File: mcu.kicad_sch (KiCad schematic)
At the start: 22 parts, among them J2 DM3CS-SF, J4 SCREEN, U4 ESP32-S3-WROOM-1U-N16R8, U8 SiP32431DR3

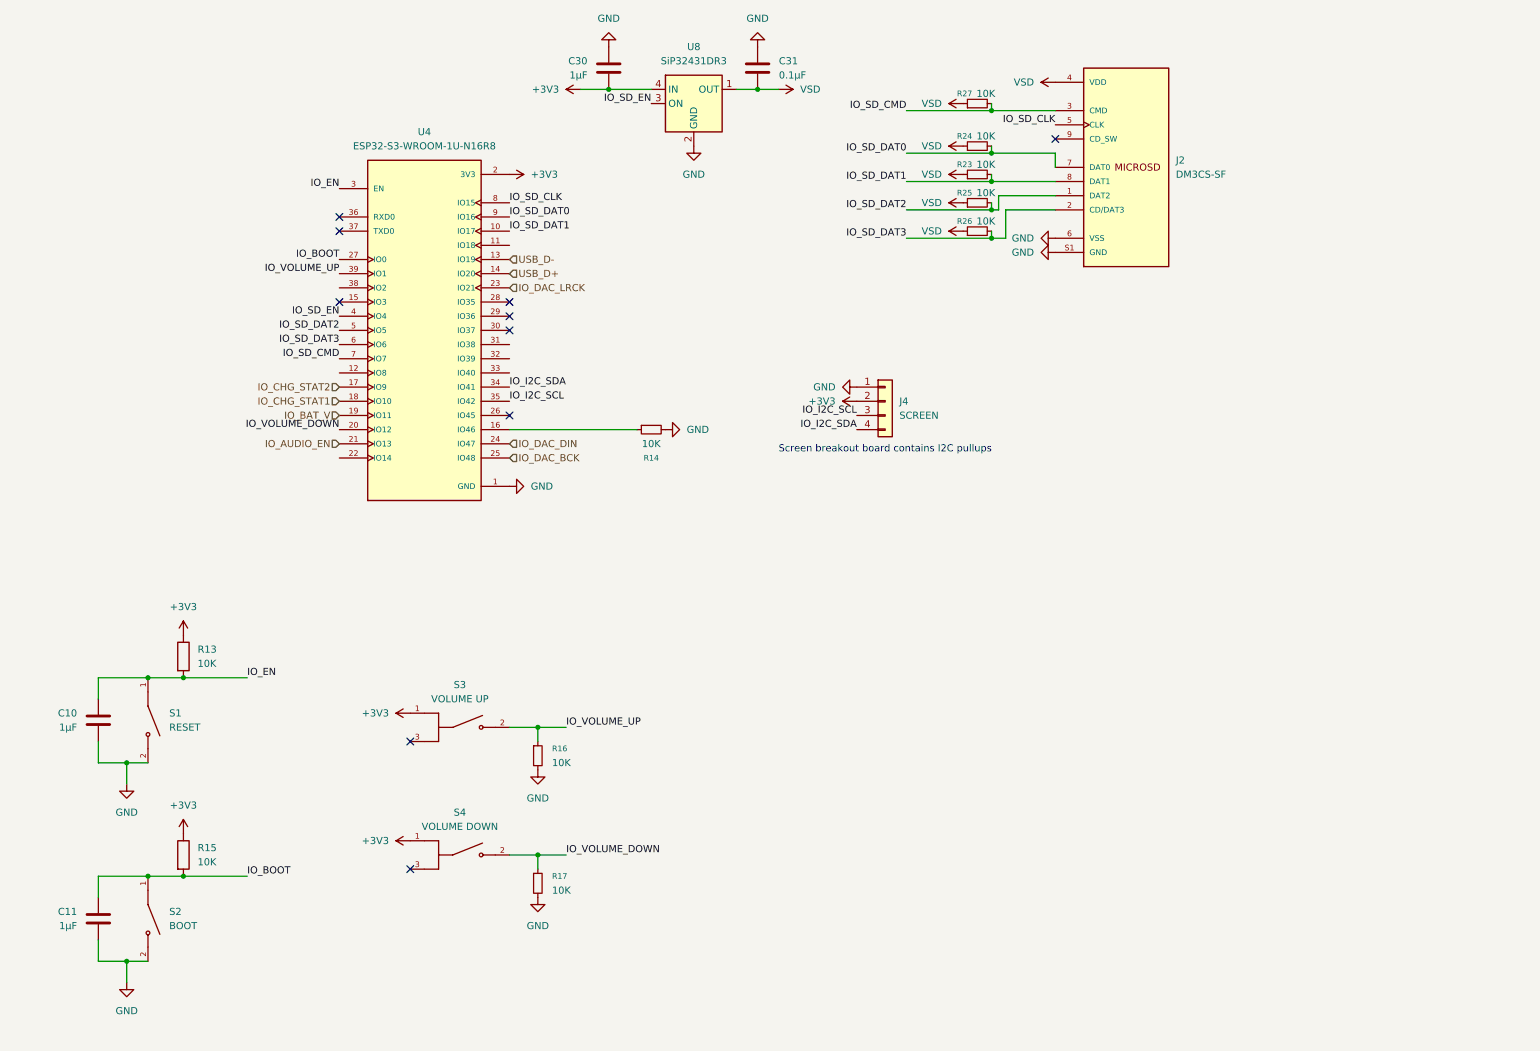
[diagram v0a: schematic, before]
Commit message: switch to stm32, wire audio section
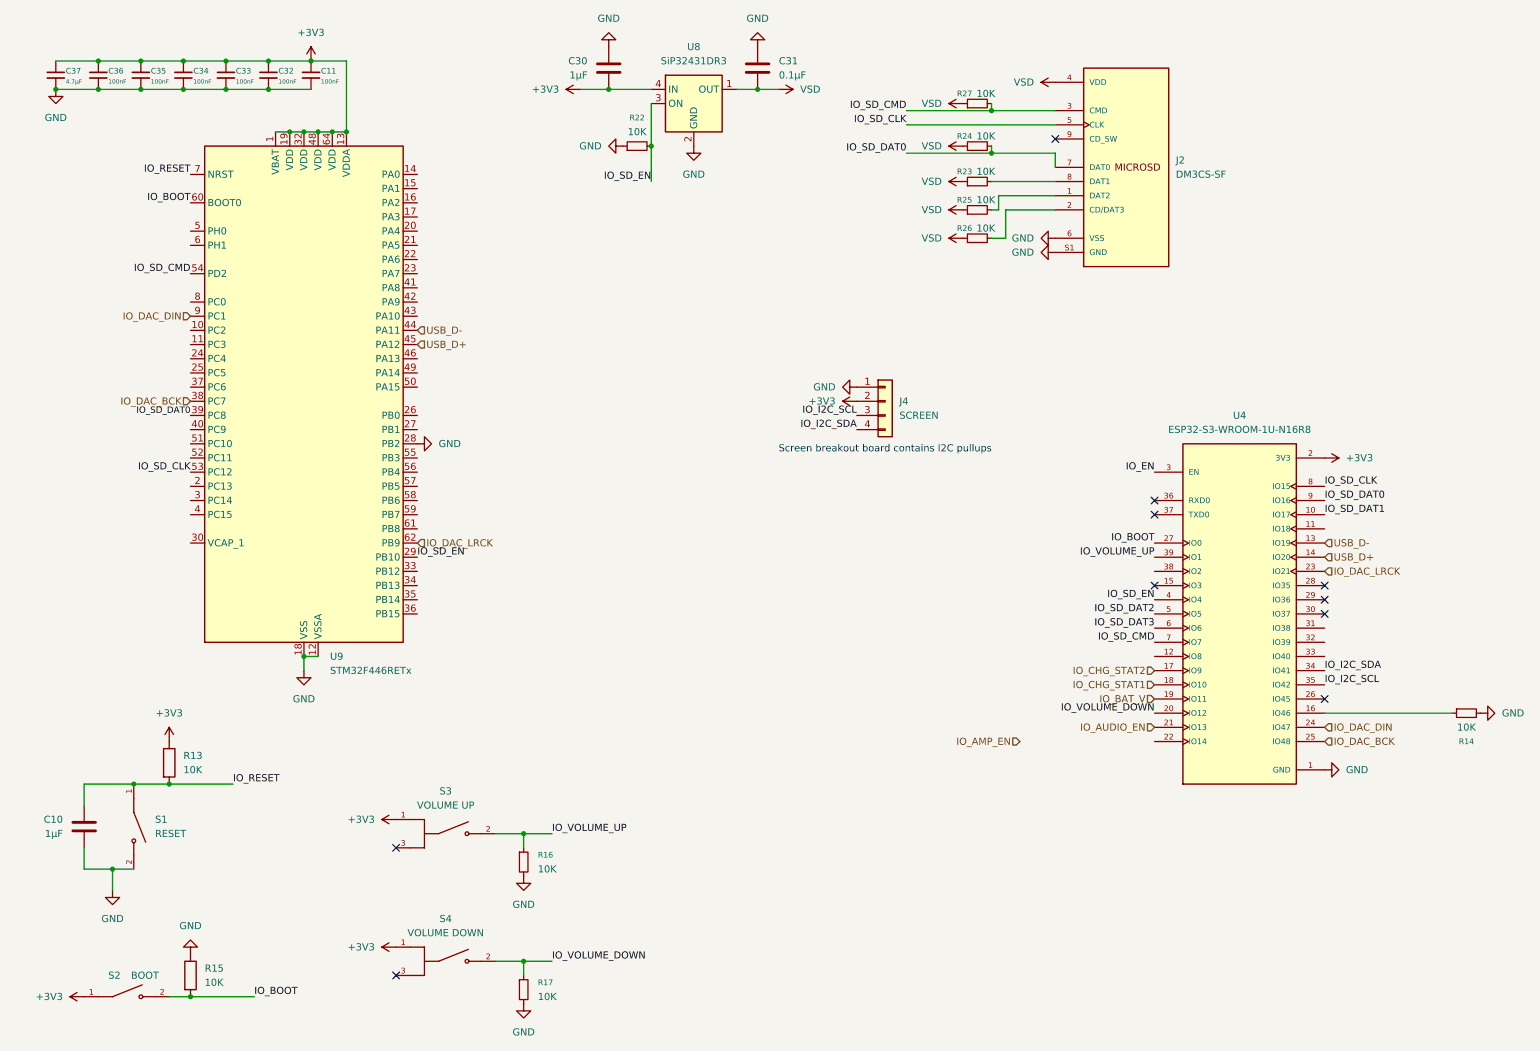
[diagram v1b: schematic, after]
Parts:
- removed C11: 1µF, Capacitor_SMD:C_0201_0603Metric, symbol Device:C
- added C11, C32, C33, C34, C35, C36: 100nF, Capacitor_SMD:C_0402_1005Metric, symbol Device:C_Small
- added C37: 4.7µF, Capacitor_SMD:C_0402_1005Metric, symbol Device:C_Small
- added R22: 10K, Resistor_SMD:R_0402_1005Metric, symbol Device:R_Small
- added U9: STM32F446RETx, Package_QFP:LQFP-64_10x10mm_P0.5mm, symbol MCU_ST_STM32F4:STM32F446RETx
- C10, C30, C31: footprint Capacitor_SMD:C_0201_0603Metric -> Capacitor_SMD:C_0402_1005Metric
- R13, R14, R15, R16, R17, R23, R24, R25, R26, R27: footprint Resistor_SMD:R_0201_0603Metric -> Resistor_SMD:R_0402_1005Metric
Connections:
- net +3V3: now also S2.1, C11.1, C32.1, C33.1, C34.1, C35.1, C36.1, C37.1, U9.1 (VBAT), U9.13 (VDDA), U9.19 (VDD), U9.32 (VDD), U9.48 (VDD), U9.64 (VDD); no longer R15.1
- net GND: now also R15.1, C11.2, C32.2, C33.2, C34.2, C35.2, C36.2, C37.2, R22.1, U9.12 (VSSA), U9.18 (VSS), U9.28 (PB2), U9.31 (VSS), U9.47 (VSS), U9.63 (VSS); no longer S2.2
- net IO_BOOT: now also S2.2, U9.60 (BOOT0); no longer S2.1
- net IO_DAC_BCK: now also U9.38 (PC7)
- net IO_DAC_DIN: now also U9.9 (PC1)
- net IO_DAC_LRCK: now also U9.62 (PB9)
- net IO_EN: no longer C10.1, R13.2, S1.1
- net IO_SD_CLK: now also U9.53 (PC12)
- net IO_SD_CMD: now also U9.54 (PD2)
- net IO_SD_DAT0: now also U9.39 (PC8)
- net IO_SD_DAT1: no longer J2.8 (DAT1), R23.2
- net IO_SD_DAT2: no longer J2.1 (DAT2), R25.2
- net IO_SD_DAT3: no longer J2.2 (CD/DAT3), R26.2
- net IO_SD_EN: now also R22.2, U9.29 (PB10)
- net USB_D+: now also U9.45 (PA12)
- net USB_D-: now also U9.44 (PA11)
- new net: J2.2 (CD/DAT3), R26.2
- new net: J2.1 (DAT2), R25.2
- new net: J2.8 (DAT1), R23.2
- new net IO_RESET: C10.1, R13.2, S1.1, U9.7 (NRST)
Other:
- moved on the sheet: C10, R13, R14, R15, R16, R17, R23, R25, R26, S1, S2, S3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

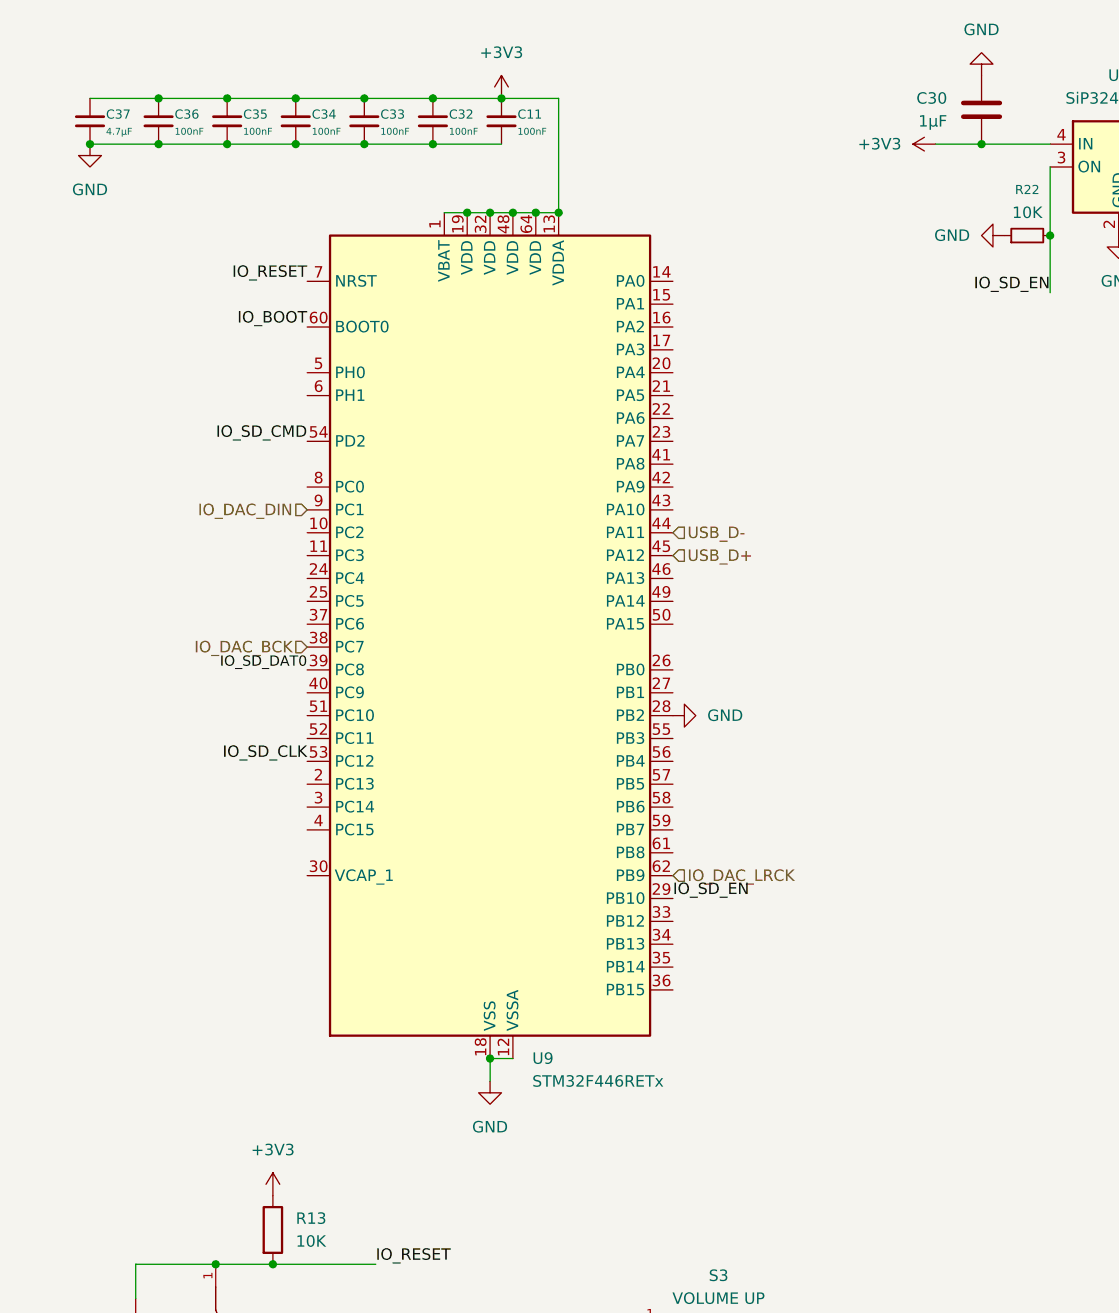
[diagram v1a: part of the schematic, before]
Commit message: add clock
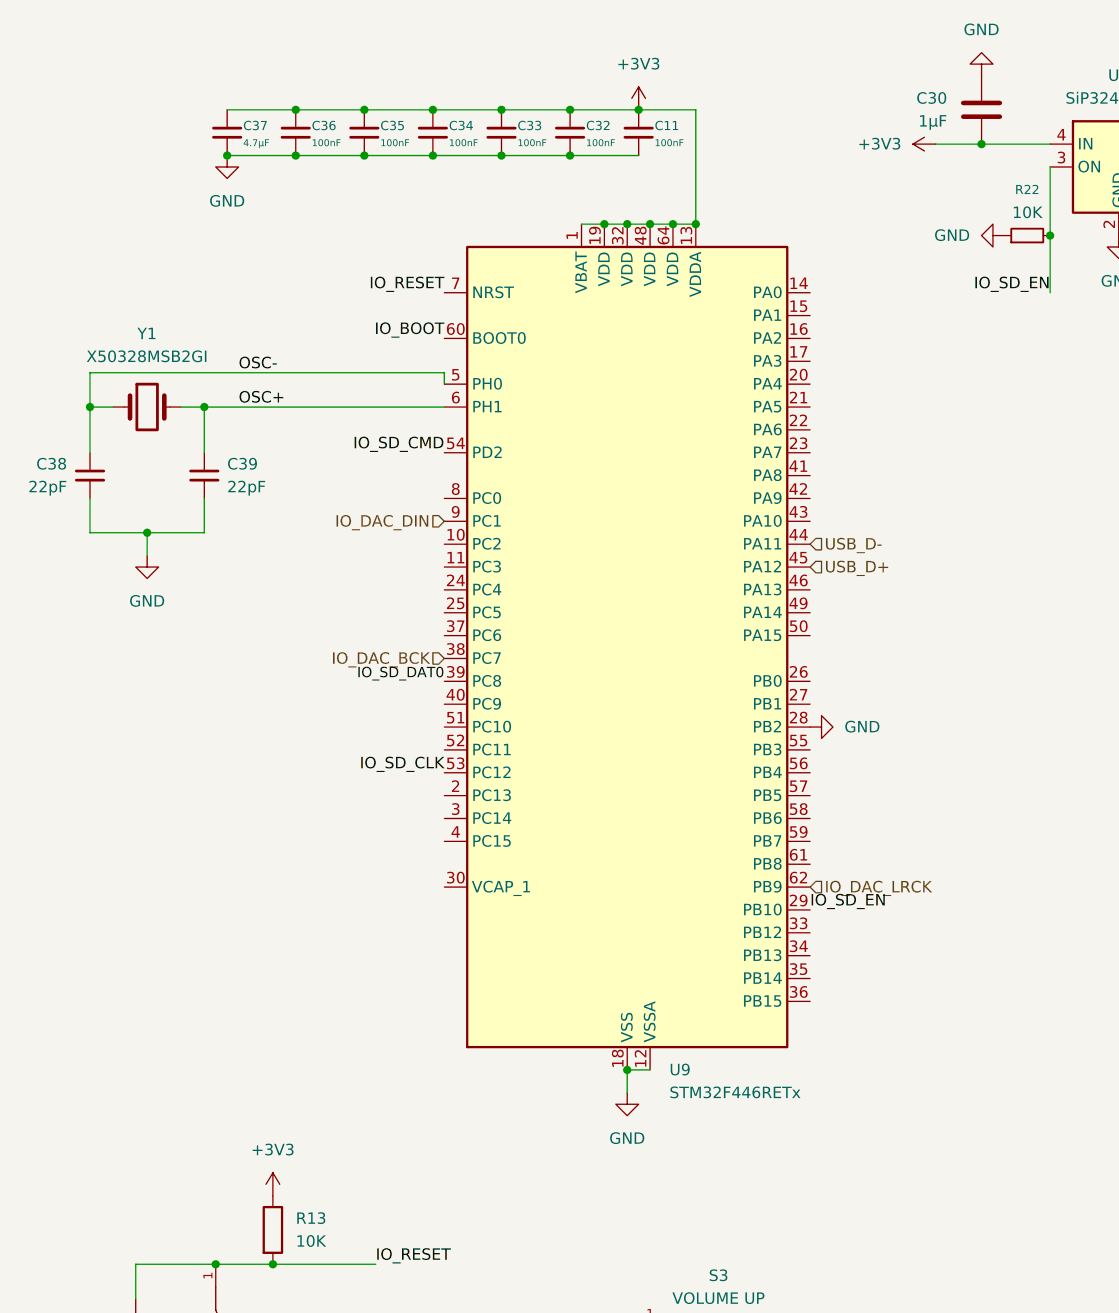
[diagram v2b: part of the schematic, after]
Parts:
- added C38, C39: 22pF, Capacitor_SMD:C_0402_1005Metric, symbol Device:C_Small
- added Y1: X50328MSB2GI, Crystal:Crystal_SMD_5032-2Pin_5.0x3.2mm, symbol Device:Crystal
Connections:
- net GND: now also C38.2, C39.2
- net OSC-: now reaches U9.5 (PH0)
- net OSC-: now also C38.1, Y1.1
- net OSC+: now reaches U9.6 (PH1)
- net OSC+: now also C39.1, Y1.2
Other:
- moved on the sheet: C11, C32, C33, C34, C35, C36, C37, U9
